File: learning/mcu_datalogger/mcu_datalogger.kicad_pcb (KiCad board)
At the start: 2 copper layers, 52.1 x 31.7 mm, 29 parts, among them J1 Conn_01x09_Pin, J2 Conn_01x04_Pin, J3 Conn_01x04_Pin, J4 Conn_02x03_Odd_Even, U1 24LC1025, U2 DS1337S_, U3 24LC1025, U4 ATMEGA328P-AU, Y1 16MHz, Y2 32.768kHz

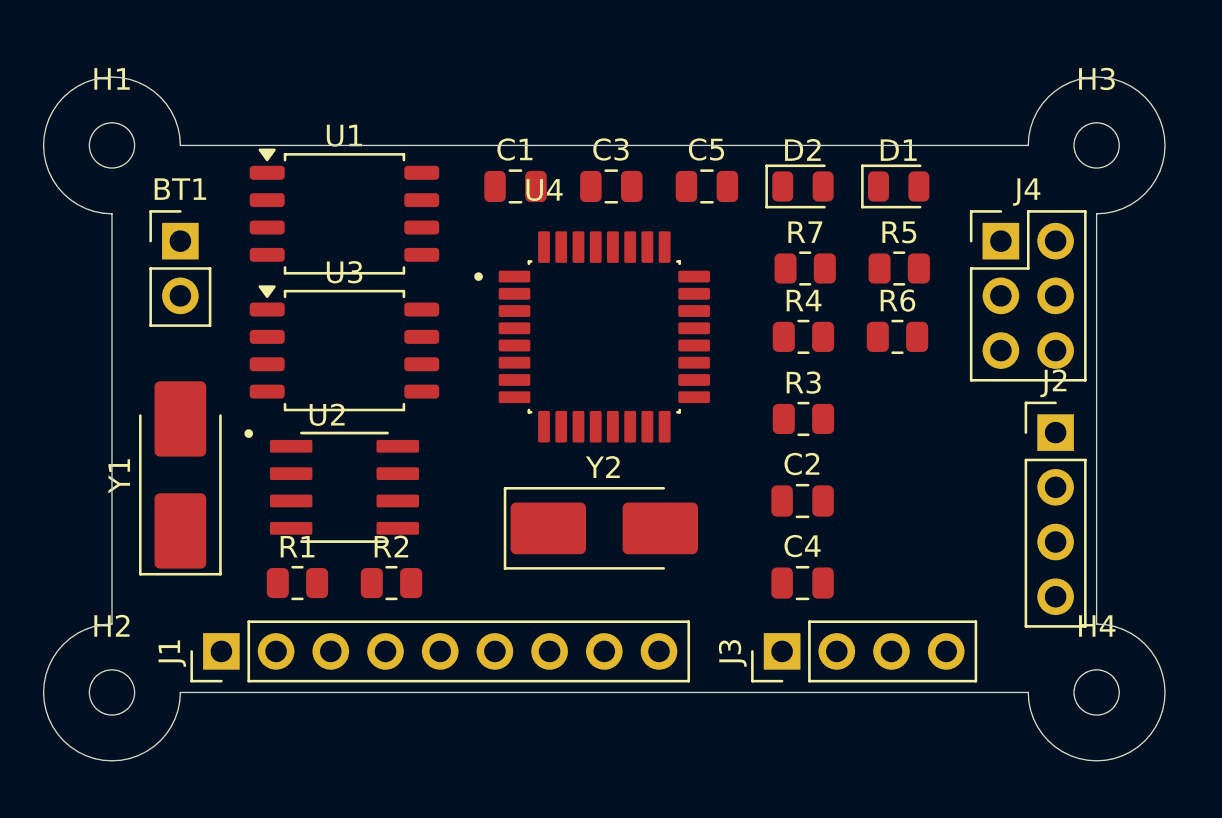
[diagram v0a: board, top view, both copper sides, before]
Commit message: Finished layout of the pcb
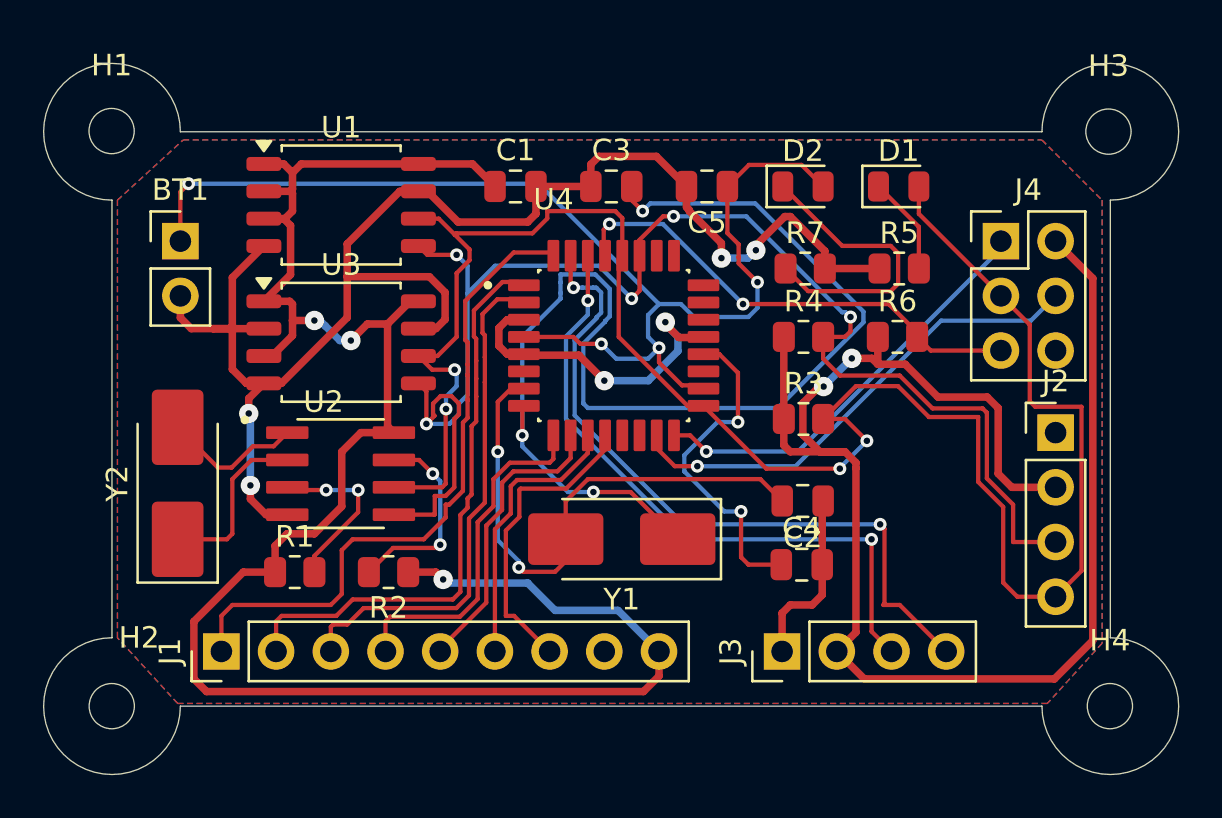
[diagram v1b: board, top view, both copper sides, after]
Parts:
- moved Y1 20.7 mm to (125.3, 91.9), turned to 180 degrees
- moved Y2 19.9 mm to (104.6, 89.3), turned to 90 degrees
- moved H4 0.88 mm to (147.9, 99.7)
- moved C4 0.85 mm to (133.6, 93.1)
- moved H3 0.84 mm to (147.9, 73.0)
- moved H1 0.67 mm to (101.6, 73.0)
- moved U2 0.66 mm to (112.2, 88.9)
- moved H2 0.64 mm to (101.6, 99.7)
- moved U4 0.59 mm to (124.9, 83.0)
- moved R2 0.53 mm to (114.4, 93.5), turned to 180 degrees
- moved R1 0.52 mm to (110.1, 93.5)
- moved U1 0.44 mm to (112.2, 76.4)
- moved U3 0.41 mm to (112.2, 82.8)
- turned C2 to 180 degrees
- turned C5 to 180 degrees
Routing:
- net /Vcc: track 0.00 -> 164.6 mm, vias 0 -> 5
- net GND: track 0.00 -> 95.9 mm, vias 0 -> 6
- net /SCK: track 0.00 -> 94.1 mm, vias 0 -> 4
- net /SDA: track 0.00 -> 67.9 mm, vias 0 -> 5
- net Net-(U4-PB7): track 0.00 -> 56.6 mm, vias 0 -> 3
- net Net-(BT1-+): track 0.00 -> 55.7 mm, vias 0 -> 4
- net /TX: track 0.00 -> 33.1 mm, vias 0 -> 2
- net /D2: track 0.00 -> 30.5 mm
- net /RX: track 0.00 -> 30.1 mm, vias 0 -> 2
- net /D3: track 0.00 -> 26.5 mm
- net Net-(U4-PB6): track 0.00 -> 25.7 mm, vias 0 -> 2
- net /D4: track 0.00 -> 23.5 mm
- net /MOSI: track 0.00 -> 22.7 mm, vias 0 -> 1
- net /RESET: track 0.00 -> 22.3 mm, vias 0 -> 2
- net /MISO: track 0.00 -> 19.7 mm, vias 0 -> 1
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- added copper zone on F.Cu, net /Vcc
- added copper zone on B.Cu, net GND
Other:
- board size 52.1 x 31.7 mm -> 52.7 x 33 mm
